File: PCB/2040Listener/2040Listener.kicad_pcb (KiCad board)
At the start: 2 copper layers, 73 x 34.5 mm, 34 parts, among them J1 CONN4_292303_SOCKET, J2 USB-AP-S-RA-PLUG, SW1 PTS815 SJM 250 SMTR LFS, SW2 PTS815 SJM 250 SMTR LFS, U1 RP2040, U2 NCP1117-3.3_SOT223, U4 BY25Q16AWTIG(R), Y1 ABM8-272-T3

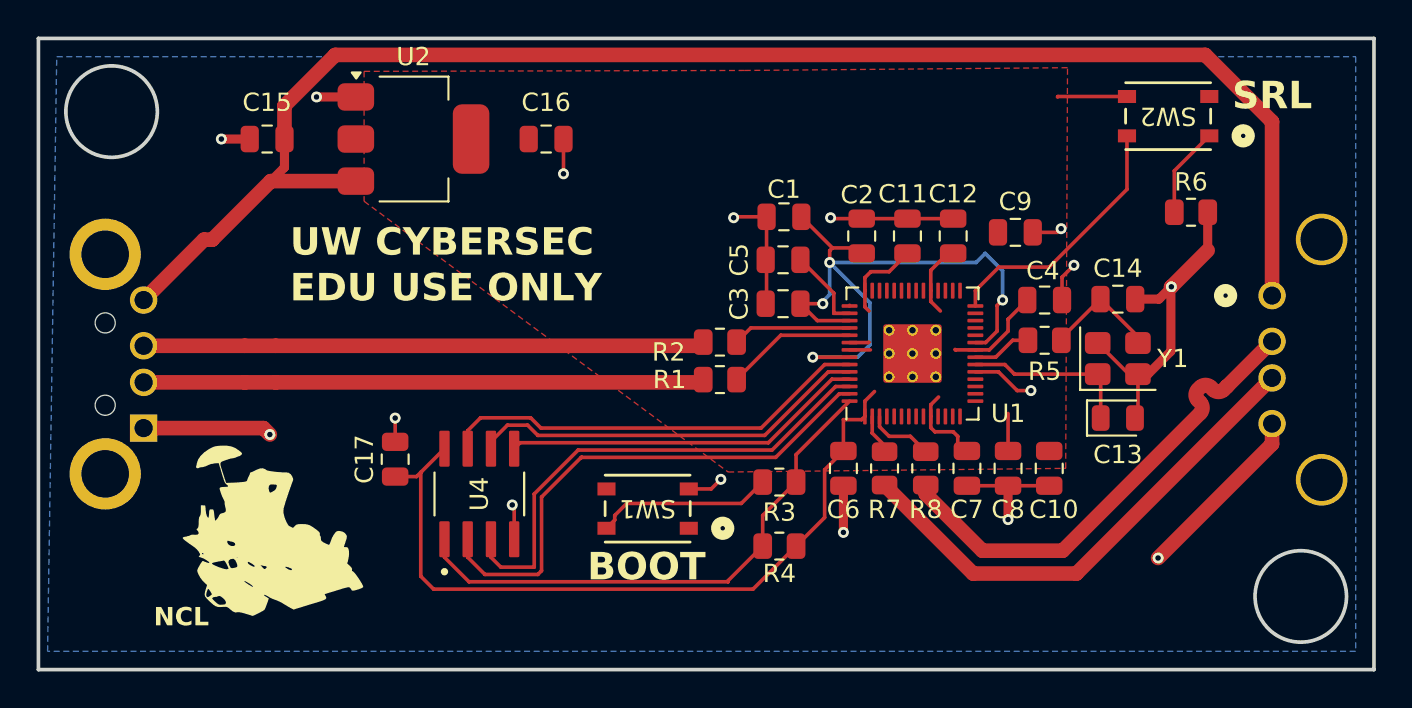
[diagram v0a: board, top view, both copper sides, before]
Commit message: pcb works!
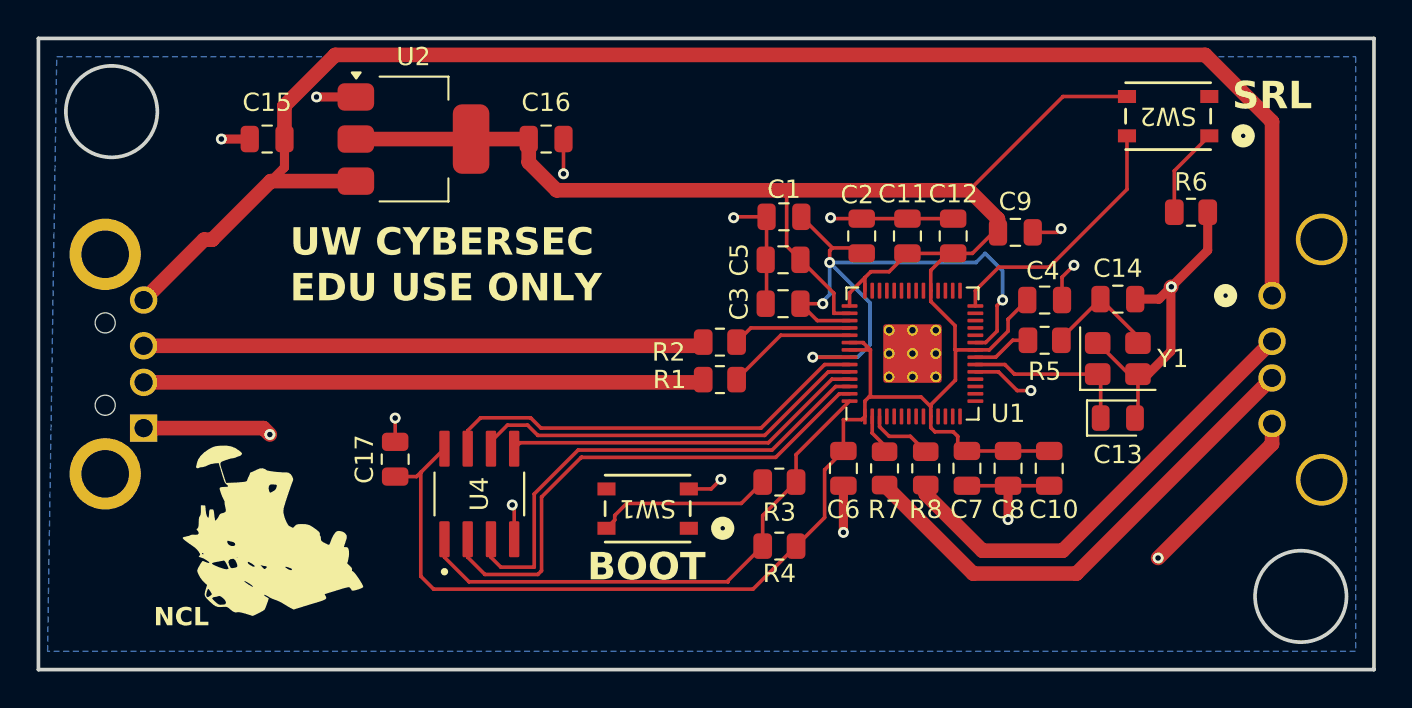
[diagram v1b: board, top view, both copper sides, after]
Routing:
- net +3V3: track 73.1 -> 142.2 mm
- net /GPIO1: track 26.7 -> 25.4 mm
- removed copper zone on F.Cu, net +3V3
